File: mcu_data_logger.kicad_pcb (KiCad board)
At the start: 2 copper layers, 48 x 34.5 mm, 29 parts, among them J1 Conn_01x04_Pin, J2 Conn_01x09_Pin, J3 Conn_01x04_Pin, J4 Conn_02x03_Odd_Even, U1 24LC1025, U2 DS1337S_, U3 24LC1025, U4 ATMEGA328P-AU, Y1 32.768 kHz, Y2 16MHz

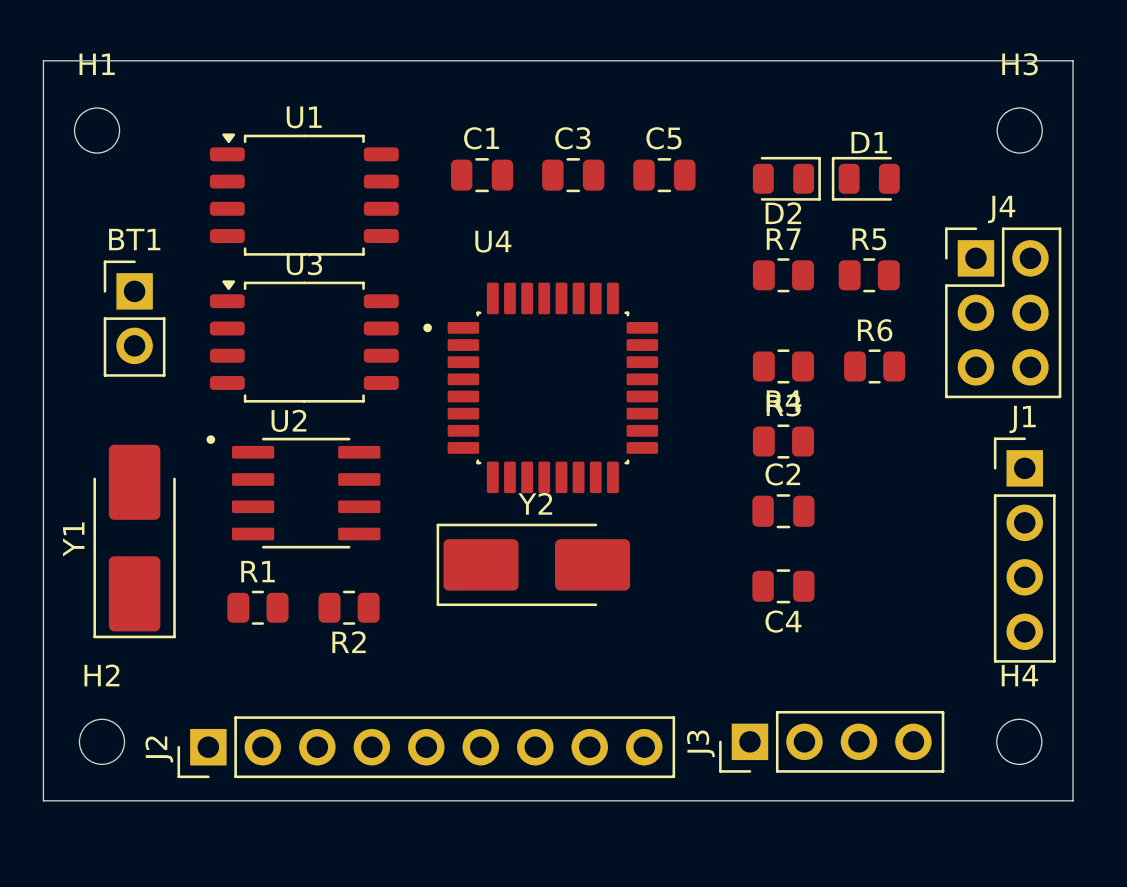
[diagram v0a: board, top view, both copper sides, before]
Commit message: initial routing done
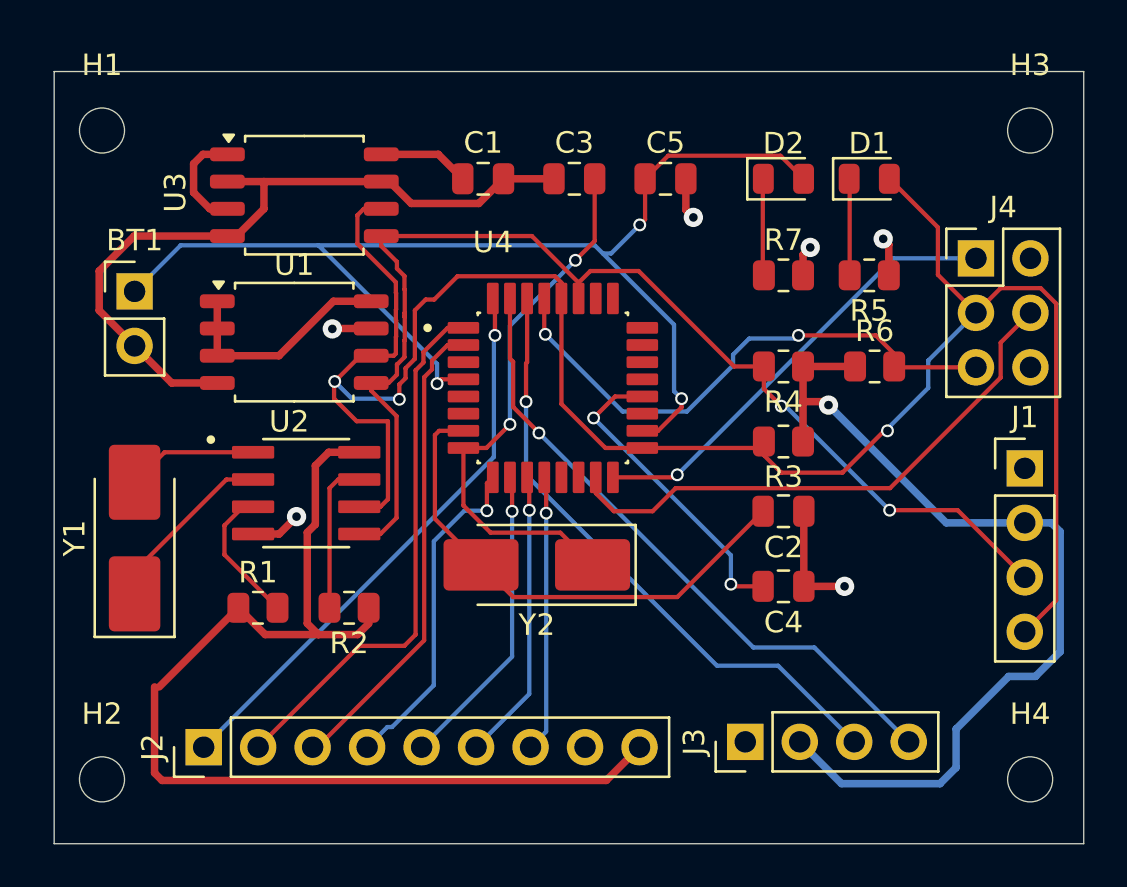
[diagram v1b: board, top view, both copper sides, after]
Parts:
- moved U1 6.87 mm to (82.7, 69.6)
- moved U3 6.85 mm to (83.2, 62.8)
- moved H4 1.82 mm to (117.0, 90.0)
- moved H2 1.75 mm to (73.7, 90.0)
- moved H3 0.48 mm to (117.0, 59.8)
- moved H1 0.23 mm to (73.7, 59.8)
- moved J2 0.22 mm to (78.5, 88.5)
- moved J3 0.22 mm to (103.7, 88.2)
- moved C1 0.18 mm to (91.5, 62.0)
- moved C3 0.18 mm to (95.8, 62.0)
- moved C5 0.18 mm to (100.0, 62.0)
- turned C2 to 180 degrees
- turned D2 to 0 degrees
- turned R3 to 180 degrees
- turned R5 to 180 degrees
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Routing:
- net /Vcc: track 0.00 -> 114.3 mm, vias 0 -> 1
- net /SCK: track 0.00 -> 95.5 mm, vias 0 -> 3
- net Net-(BT1-+): track 0.00 -> 56.7 mm, vias 0 -> 3
- net /SDA: track 0.00 -> 55.7 mm, vias 0 -> 2
- net GND: track 0.00 -> 50.4 mm, vias 0 -> 6
- net /TX: track 0.00 -> 30.0 mm, vias 0 -> 1
- net /RX: track 0.00 -> 28.7 mm, vias 0 -> 1
- net /D2: track 0.00 -> 26.6 mm, vias 0 -> 1
- net /MOSI: track 0.00 -> 26.1 mm
- net /RESET: track 0.00 -> 26.0 mm, vias 0 -> 2
- net Net-(U4-PB7): track 0.00 -> 25.6 mm, vias 0 -> 2
- net /D3: track 0.00 -> 25.2 mm
- net Net-(U4-PB6): track 0.00 -> 23.8 mm
- net /D4: track 0.00 -> 22.2 mm
- net /MISO: track 0.00 -> 21.2 mm, vias 0 -> 1
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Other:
- board size 48 x 34.5 mm -> 48 x 36 mm
